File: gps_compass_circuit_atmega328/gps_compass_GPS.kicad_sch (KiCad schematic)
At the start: 5 parts, among them U1 LSM303C, U2 MAX-M8C

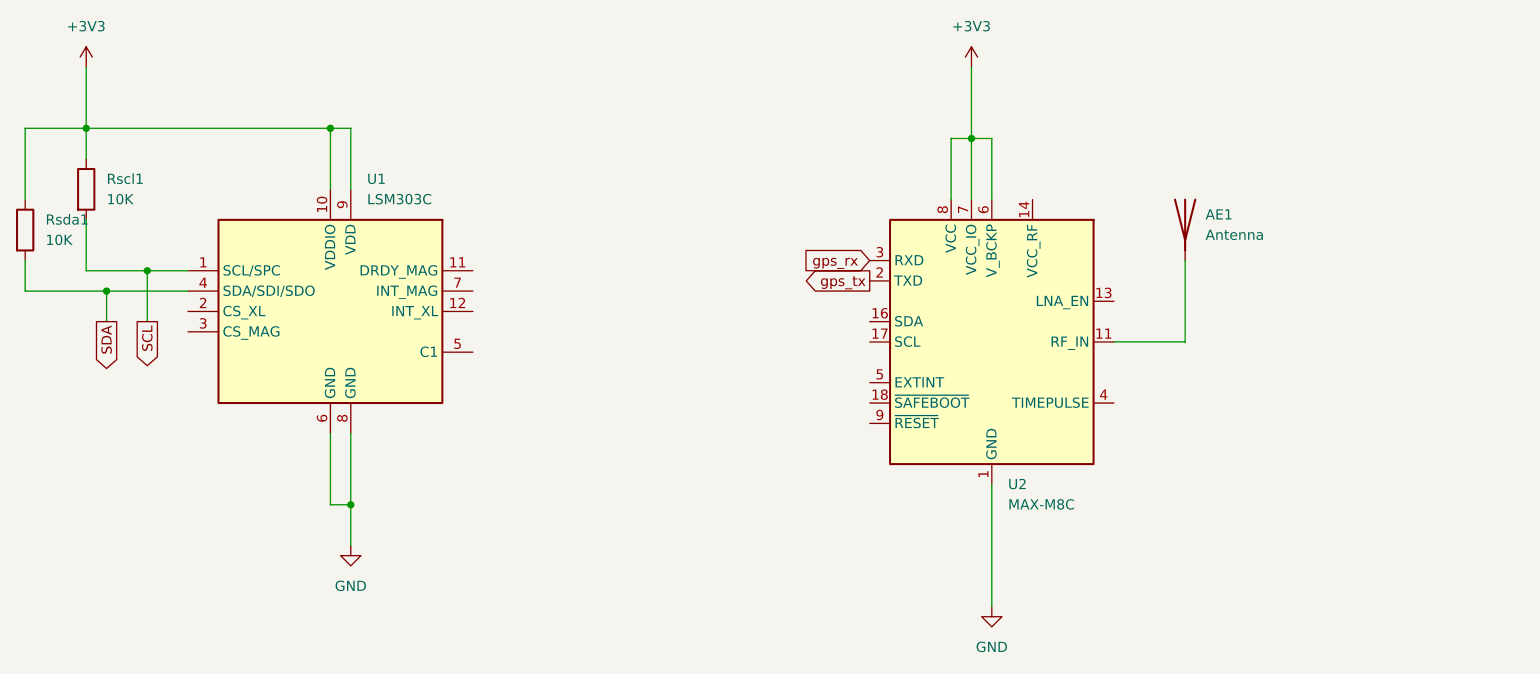
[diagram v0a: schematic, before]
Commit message: upd circuit
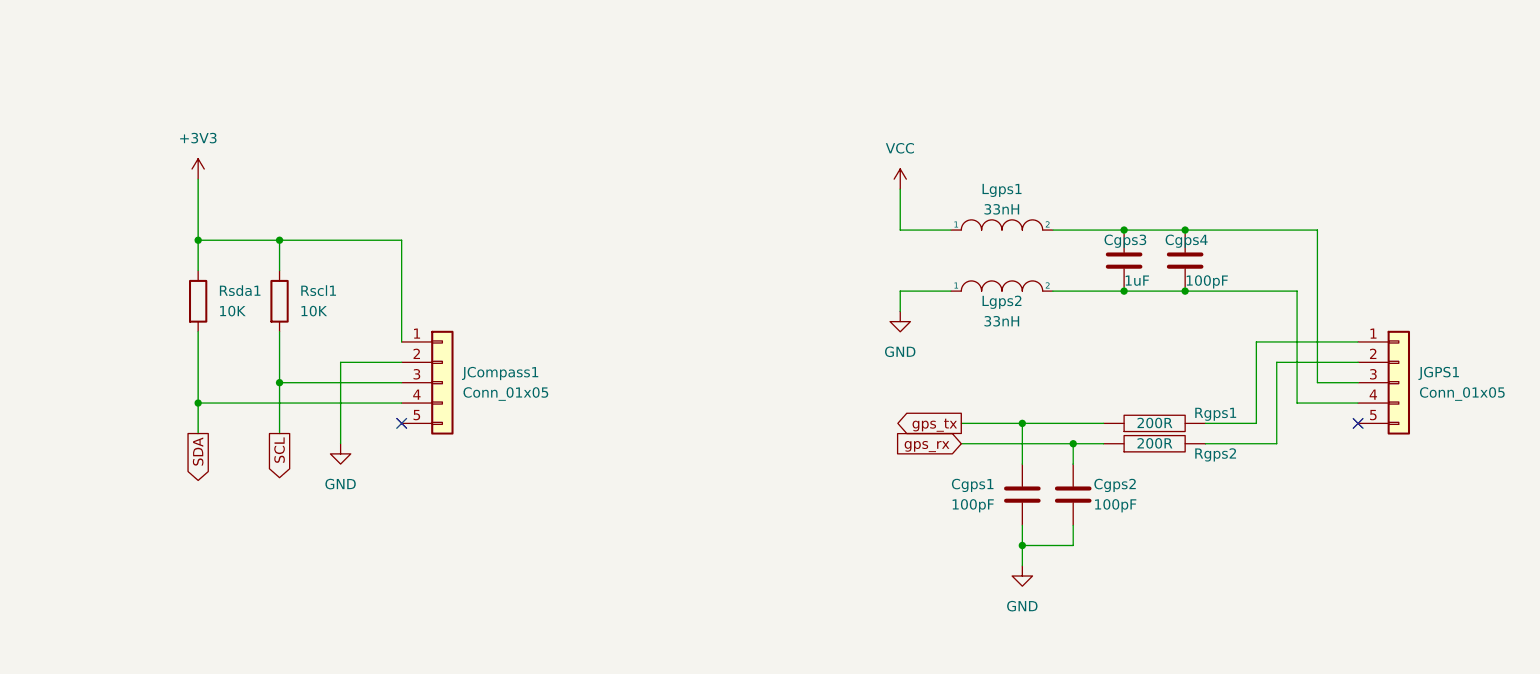
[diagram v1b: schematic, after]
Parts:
- removed AE1: Antenna, Connector_Coaxial:U.FL_Hirose_U.FL-R-SMT-1_Vertical, symbol Device:Antenna
- removed U1: LSM303C, Package_LGA:LGA-12_2x2mm_P0.5mm, symbol Sensor_Motion:LSM303C
- removed U2: MAX-M8C, RF_GPS:ublox_MAX, symbol RF_GPS:MAX-M8C
- added Cgps1, Cgps2, Cgps4: 100pF, Capacitor_SMD:C_0603_1608Metric, symbol Device:C
- added Cgps3: 1uF, Capacitor_SMD:C_0603_1608Metric, symbol Device:C
- added JCompass1, JGPS1: Conn_01x05, Connector_PinSocket_2.54mm:PinSocket_1x05_P2.54mm_Vertical, symbol Connector_Generic:Conn_01x05
- added Lgps1, Lgps2: 33nH, Inductor_SMD:L_0603_1608Metric, symbol pspice:INDUCTOR
- added Rgps1, Rgps2: 200R, Resistor_SMD:R_0603_1608Metric, symbol pspice:R
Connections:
- net +3V3: now also JCompass1.1 (Pin_1)
- net GND: now also Cgps1.2, Cgps2.2, JCompass1.2 (Pin_2), Lgps2.1
- net SCL: now also JCompass1.3 (Pin_3)
- net SDA: now also JCompass1.4 (Pin_4)
- net gps_rx: now also Cgps2.1, Rgps2.1
- net gps_tx: now also Cgps1.1, Rgps1.1
- new net: Cgps3.1, Cgps4.1, JGPS1.3 (Pin_3), Lgps1.2
- new net: JGPS1.1 (Pin_1), Rgps1.2
- new net: JGPS1.2 (Pin_2), Rgps2.2
- new net: Cgps3.2, Cgps4.2, JGPS1.4 (Pin_4), Lgps2.2
- new net VCC: Lgps1.1
- no-connect marks 0 -> 2
